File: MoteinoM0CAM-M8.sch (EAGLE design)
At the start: 17 parts

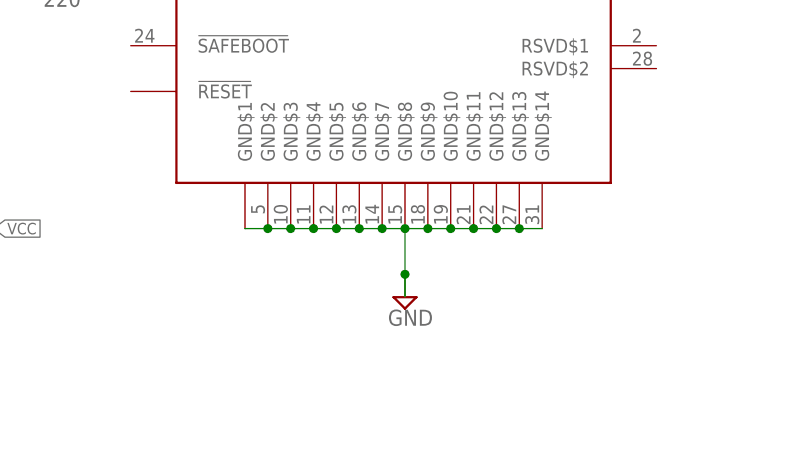
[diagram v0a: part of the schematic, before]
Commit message: Connection tidy, layout tweaks
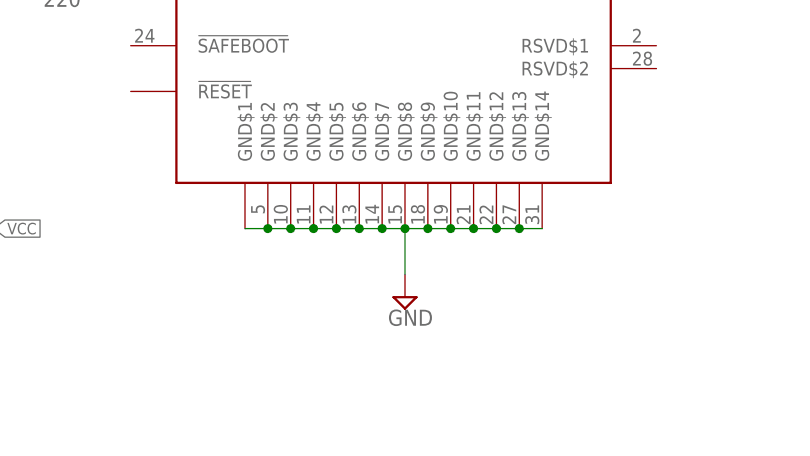
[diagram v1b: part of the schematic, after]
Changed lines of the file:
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@@
 <wire x1="119.38" y1="111.76" x2="119.38" y2="106.68" width="0.1524" layer="91"/>
 <pinref part="SUPPLY33" gate="GND" pin="GND"/>
-<wire x1="119.38" y1="106.68" x2="119.38" y2="104.14" width="0.1524" layer="91"/>
-<junction x="119.38" y="106.68"/>
 </segment>
 <segment>
